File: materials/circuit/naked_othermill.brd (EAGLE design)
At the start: 91.1 x 80 mm, 20 parts, among them IC1 LM358N

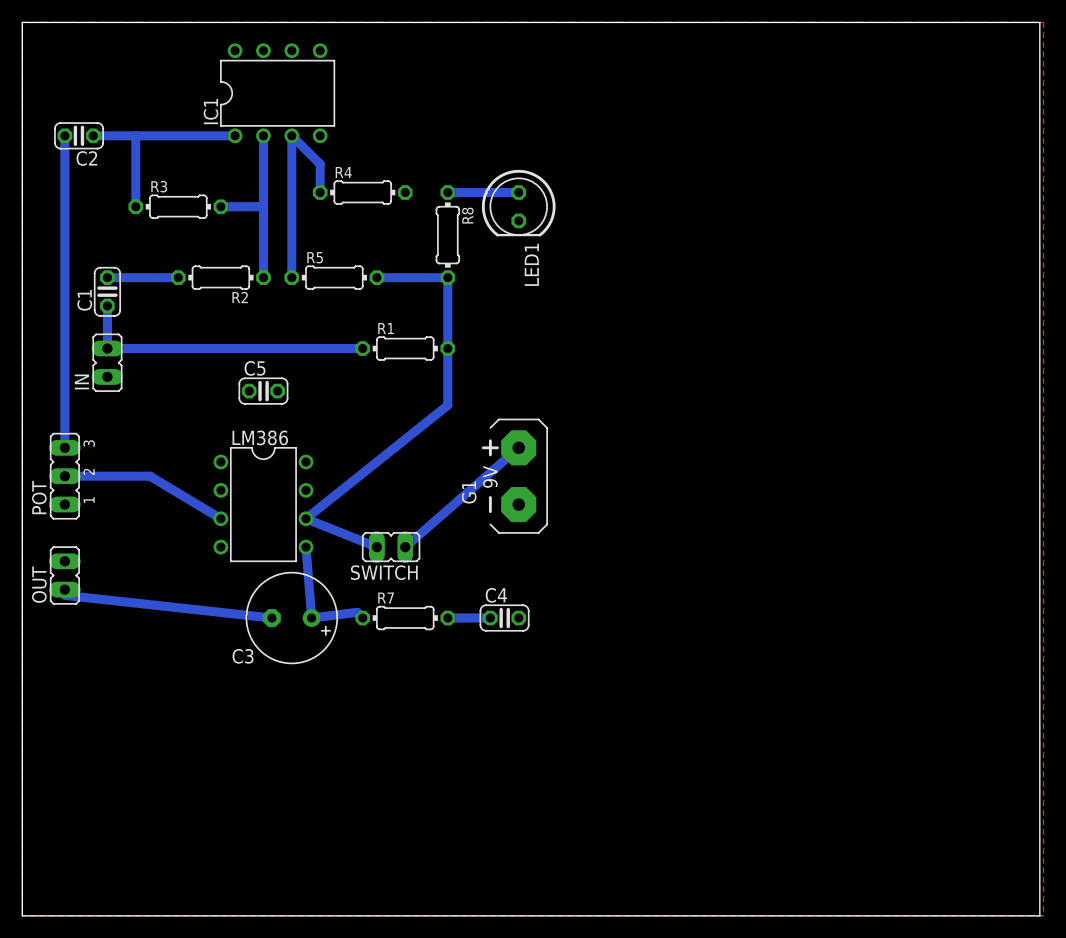
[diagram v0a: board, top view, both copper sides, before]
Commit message: updates with othermill and references
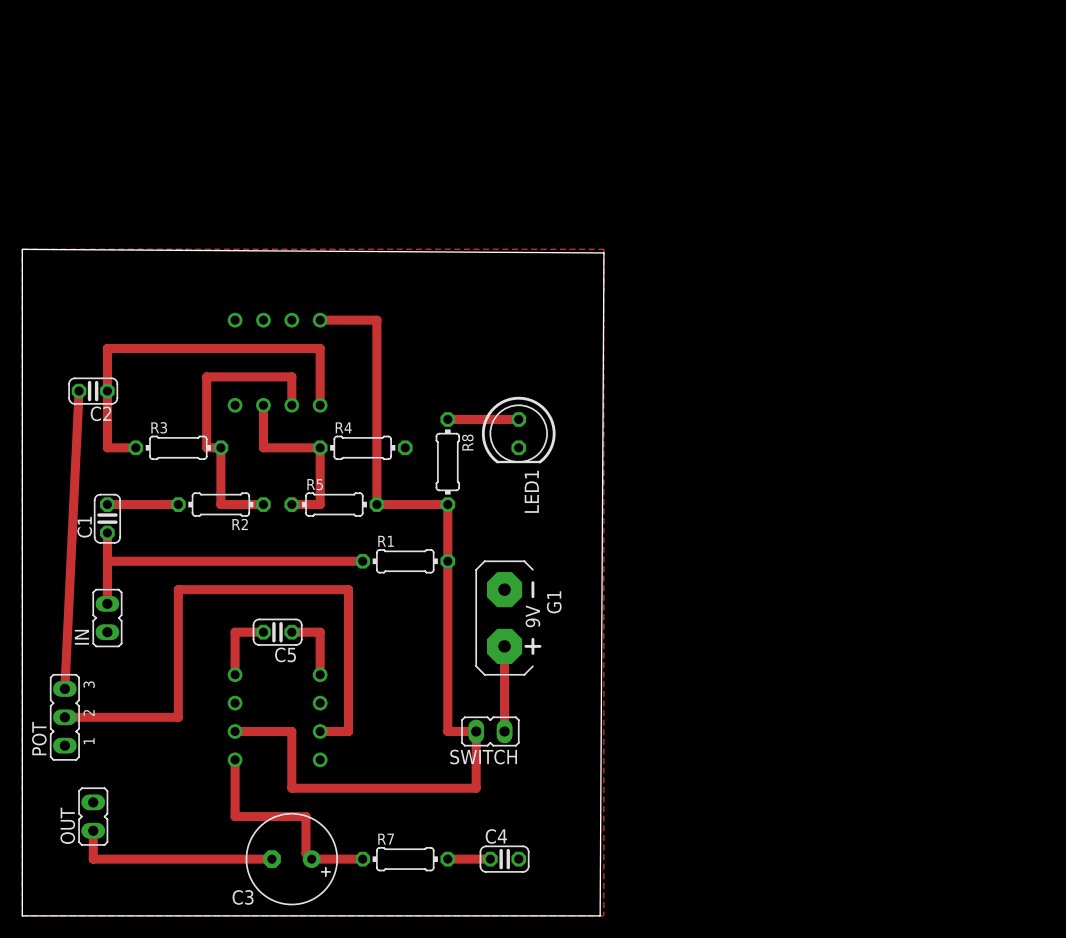
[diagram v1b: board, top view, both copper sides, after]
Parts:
- moved IC1 24.1 mm to (22.9, 49.5), flipped to the bottom
- moved C2 22.9 mm to (6.35, 47.0)
- moved IN 22.9 mm to (7.62, 26.7)
- moved R4 22.9 mm to (30.5, 41.9)
- moved OUT 21.7 mm to (6.35, 8.89)
- moved C5 21.6 mm to (22.9, 25.4), turned to 180 degrees
- moved C3 21.6 mm to (24.1, 5.08)
- moved C4 21.6 mm to (43.2, 5.08)
- moved R3 21.6 mm to (14.0, 41.9)
- moved R7 21.6 mm to (34.3, 5.08)
- moved POT 21.6 mm to (3.81, 17.8)
- moved C1 20.3 mm to (7.62, 35.6)
- moved LED1 20.3 mm to (44.5, 43.2)
- moved R2 20.3 mm to (17.8, 36.8)
- moved R5 20.3 mm to (27.9, 36.8)
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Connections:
- removed net V+: IC1.8
- net 9V: now also IC1.8
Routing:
- net 9V: track 40.9 -> 82.5 mm
- net N$9: track 15.0 -> 52.1 mm
- net N$7: track 19.0 -> 35.6 mm
- net N$4: track 16.5 -> 26.7 mm
- net N$10: track 11.2 -> 20.0 mm
- net N$5: track 0.00 -> 6.35 mm
- net N$14: track 0.00 -> 6.35 mm
- net N$1: track 13.5 -> 7.62 mm
- net N$2: track 26.7 -> 29.2 mm
- net N$6: track 18.8 -> 16.5 mm
- net N$8: track 27.9 -> 26.7 mm
- net N$11: track 19.2 -> 18.5 mm
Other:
- board size 91.1 x 80 mm -> 52.1 x 59.7 mm
